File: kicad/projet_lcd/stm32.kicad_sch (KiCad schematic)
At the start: 36 parts, among them U1 STM32H563ZIT6, Y1 25MHZ, Y2 32.768KHZ

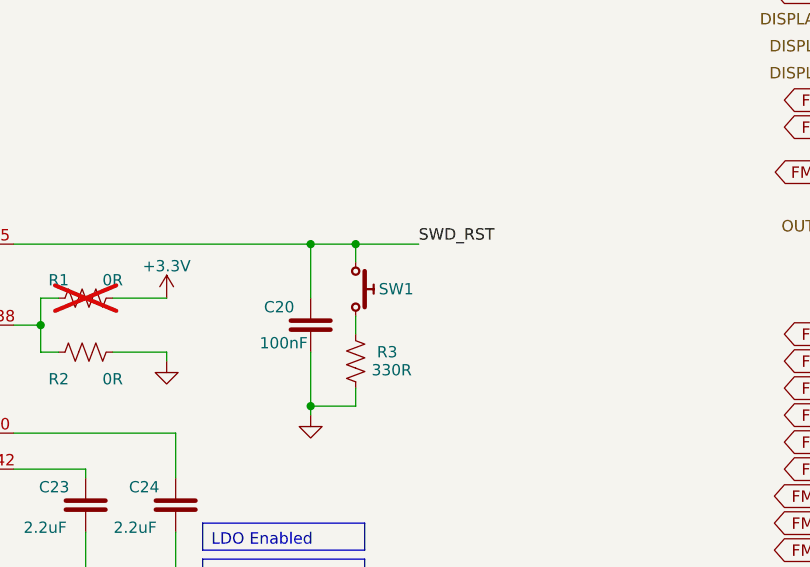
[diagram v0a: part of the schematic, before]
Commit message: schematiks seems okayish
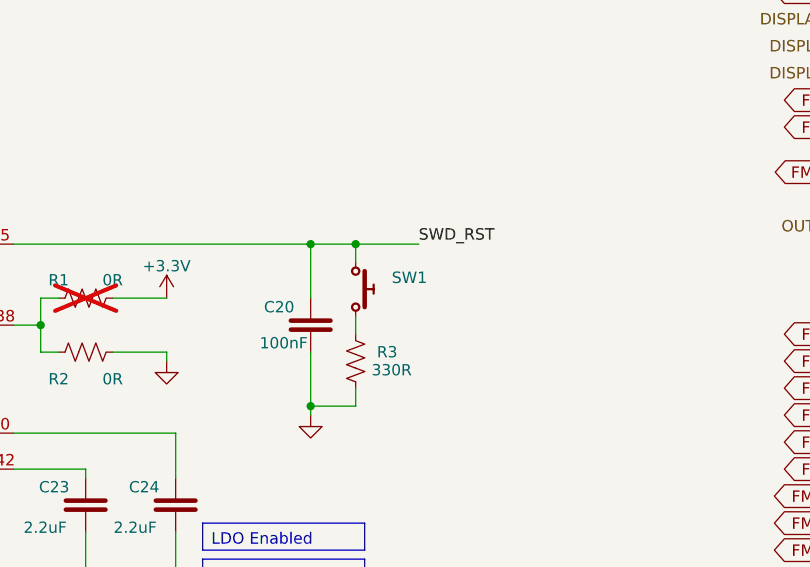
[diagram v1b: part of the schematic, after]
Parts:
- removed SW1: ~, symbol Generics:SW_PushButton
- added SW1: ~, Misc:C284397, symbol Misc:sw_C2844397
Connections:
- net SWD_RST: now also SW1.1, SW1.2
- net at R3.2 (1): now also SW1.3, SW1.4
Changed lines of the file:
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@@
 	)
 	(symbol
+		(lib_id "Misc:sw_C2844397")
+		(at 201 76 270)
+		(unit 1)
+		(exclude_from_sim no)
+		(in_bom yes)
+		(on_board yes)
+		(dnp no)
+		(fields_autoplaced yes)
+		(property "Reference" "SW1"
+			(at 205.01 77.7299 90)
+			(effects
+				(font
+					(size 1.27 1.27)
+				)
+				(justify left)
+			)
+		)
+		(property "Value" "~"
+			(at 205.01 80.2699 90)
+			(effects
+				(font
+					(size 1.27 1.27)
+				)
+				(justify left)
+				(hide yes)
+			)
+		)
+		(property "Footprint" "Misc:C284397"
+			(at 208.5 79.5 0)
+			(effects
+				(font
+					(size 1.27 1.27)
+				)
+				(hide yes)
+			)
+		)
+		(property "Datasheet" ""
+			(at 201 76 0)
+			(effects
+				(font
+					(size 1.27 1.27)
+				)
+				(hide yes)
+			)
+		)
+		(property "Description" "Switch SPST"
+			(at 206 80 0)
+			(effects
+				(font
+					(size 1.27 1.27)
+				)
+				(hide yes)
+			)
+		)
+		(property "LCSC Part #" "C2844397"
+			(at 210.5 79.5 0)
+			(effects
+				(font
+					(size 1.27 1.27)
+				)
+				(hide yes)
+			)
+		)
+		(pin "3"
+		)
+		(pin "4"
+		)
+		(pin "2"
+		)
+		(pin "1"
+		)
+		(instances
+			(project ""
+				(path "/b3ce22de-813e-4a84-80c2-bec39c904000/9ea47d51-491e-4a8f-867a-699065ac1e83"
+					(reference "SW1")
+					(unit 1)
+				)
+			)
+		)
+	)
+	(symbol
 		(lib_id "Generics:C")
 		(at 47 37 90)
@@
 					(unit 1)
 				)
-			)
-		)
-	)
-	(symbol
-		(lib_id "Generics:SW_PushButton")
-		(at 201 76 270)
-		(unit 1)
-		(exclude_from_sim no)
-		(in_bom yes)
-		(on_board yes)
-		(dnp no)
-		(property "Reference" "SW1"
-			(at 205.5 79 90)
-			(do_not_autoplace yes)
-			(effects
-				(font
-					(size 1.25 1.25)
-				)
-			)
-		)
-		(property "Value" "~"
-			(at 190 80 0)
-			(effects
-				(font
-					(size 1.25 1.25)
-				)
-				(hide yes)
-			)
-		)
-		(property "Footprint" ""
-			(at 206.08 81 0)
-			(effects
-				(font
-					(size 1.25 1.25)
-				)
-				(hide yes)
-			)
-		)
-		(property "Datasheet" ""
-			(at 188 80 0)
-			(effects
-				(font
-					(size 1.25 1.25)
-				)
-				(hide yes)
-			)
-		)
-		(property "Description" "Push button switch, generic, two pins"
-			(at 197.1 79 0)
-			(effects
-				(font
-					(size 1.25 1.25)
-				)
-				(hide yes)
-			)
-		)
-		(property "Part#" ""
-			(at 201 76 0)
-			(effects
-				(font
-					(size 1.25 1.25)
-				)
-				(hide yes)
-			)
-		)
-		(property "Comments" ""
-			(at 201 76 0)
-			(effects
-				(font
-					(size 1.25 1.25)
-				)
-				(hide yes)
-			)
-		)
-		(pin "1"
-		)
-		(pin "2"
-		)
-		(instances
-			(project ""
-				(path "/b3ce22de-813e-4a84-80c2-bec39c904000/9ea47d51-491e-4a8f-867a-699065ac1e83"
-					(reference "SW1")
-					(unit 1)
-				)
